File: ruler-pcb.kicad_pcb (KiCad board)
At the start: 2 copper layers, 202 x 51 mm, 58 parts

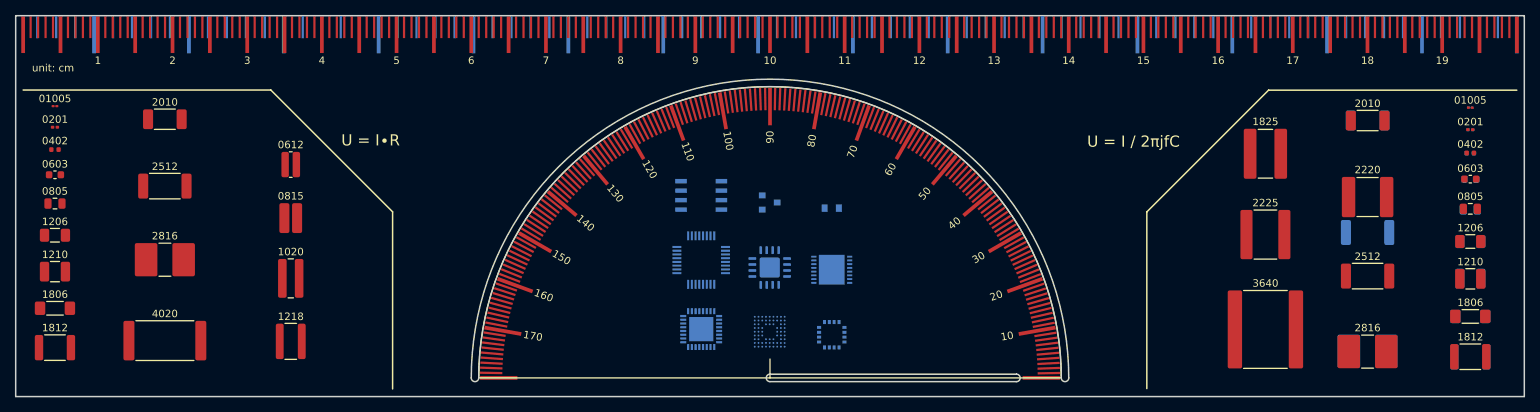
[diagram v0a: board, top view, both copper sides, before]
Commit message: ready to fab
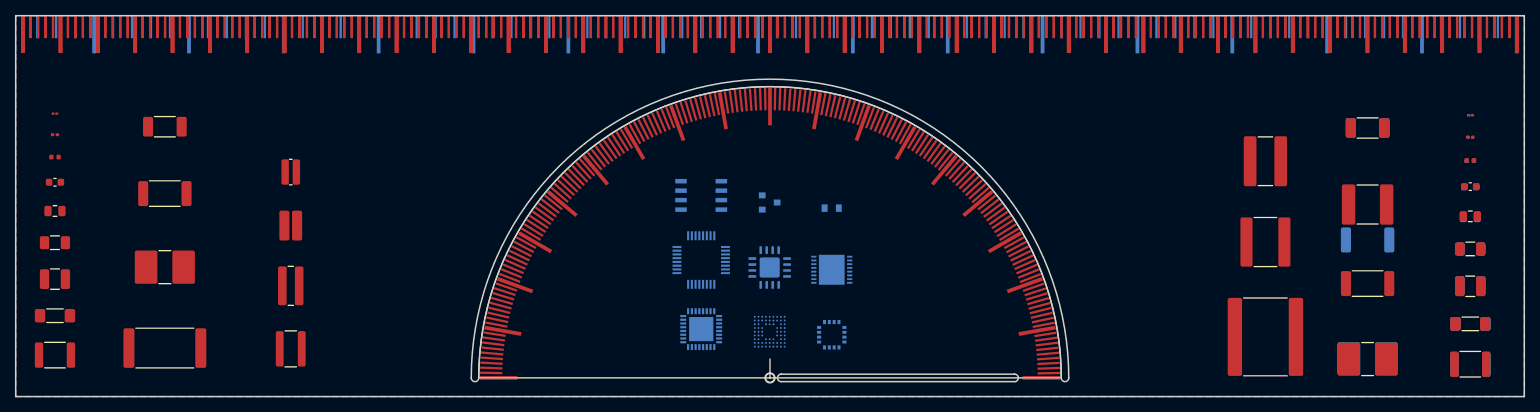
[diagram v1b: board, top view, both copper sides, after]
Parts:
- added G***: LOGO, LOGO, B.Cu at (57.1, 58.0)
- added REF**: ruler-20-cm, Ruler:ruler-20-cm, F.Cu at (25.4, 75.7)
- REF**: footprint Symbol:Symbol_KiCAD-Logo_CopperAndSilkScreenTop -> Symbol:KiCad-Logo_5mm_SolderMask
- moved REF** 23.3 mm to (33.1, 70.7)
- moved 01005 1.00 mm to (29.7, 38.8)
- moved 01005 1.00 mm to (219.2, 39.0) (x2)
- moved 0201 1.00 mm to (29.7, 41.6)
- moved 0201 1.00 mm to (219.2, 42.0) (x2)
- moved 0402 1.00 mm to (29.7, 44.6)
- moved 0402 1.00 mm to (219.2, 45.1) (x2)
- moved 0603 1.00 mm to (29.7, 48.0)
- moved 0603 1.00 mm to (219.2, 48.6) (x2)
- moved 0612 1.00 mm to (61.2, 46.6)
- moved 0805 1.00 mm to (29.7, 51.9)
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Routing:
- net (no net): vias 0 -> 1
- added copper zone on B.Cu, net (none)
- added copper zone on F.Cu, net (none)
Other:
- outline, holes or cut-outs redrawn
- board text added: "01005"
- board text added: "0201"
- board text added: "0402"
- board text added: "0603"
- board text added: "0612"
- board text added: "0805"
- board text added: "0815"
- board text added: "1"
- board text added: "10"
- board text added: "100"
- board text added: "1020"
- board text added: "11"
- board text added: "110"
- board text added: "12"
- board text added: "120"
- board text added: "1206"
- board text added: "1210"
- board text added: "1218"
- board text added: "13"
- board text added: "130"
- board text added: "14"
- board text added: "140"
- board text added: "15"
- board text added: "150"
- board text added: "16"
- board text added: "160"
- board text added: "17"
- board text added: "170"
- board text added: "18"
- board text added: "1806"
- board text added: "1812"
- board text added: "1825"
- board text added: "19"
- board text added: "2"
- board text added: "20"
- board text added: "2010"
- board text added: "2220"
- board text added: "2225"
- board text added: "2512"
- board text added: "2816"
- board text added: "3"
- board text added: "30"
- board text added: "3640"
- board text added: "4"
- board text added: "40"
- board text added: "4020"
- board text added: "5"
- board text added: "50"
- board text added: "6"
- board text added: "60"
- board text added: "7"
- board text added: "70"
- board text added: "8"
- board text added: "80"
- board text added: "9"
- board text added: "90"
- board text added: "BGA"
- board text added: "DFN"
- board text added: "LFCSP"
- board text added: "LGA"
- board text added: "LQFP"
- board text added: "QFN"
- board text added: "SOD"
- board text added: "SOIC"
- board text added: "SOT"
- board text added: "unit: cm"
- board text added: "unit: inch"
